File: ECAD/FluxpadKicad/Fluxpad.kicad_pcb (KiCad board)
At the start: 2 copper layers, 39 x 60 mm, 26 parts, among them SW1 SW_SPST, SW2 SW_SPST, SW3 PEC12R-4017F-N0024, U1 SeeeduinoXIAO, U2 DRV5056A3QDBZx Lekker, U3 DRV5056A3QDBZx Lekker

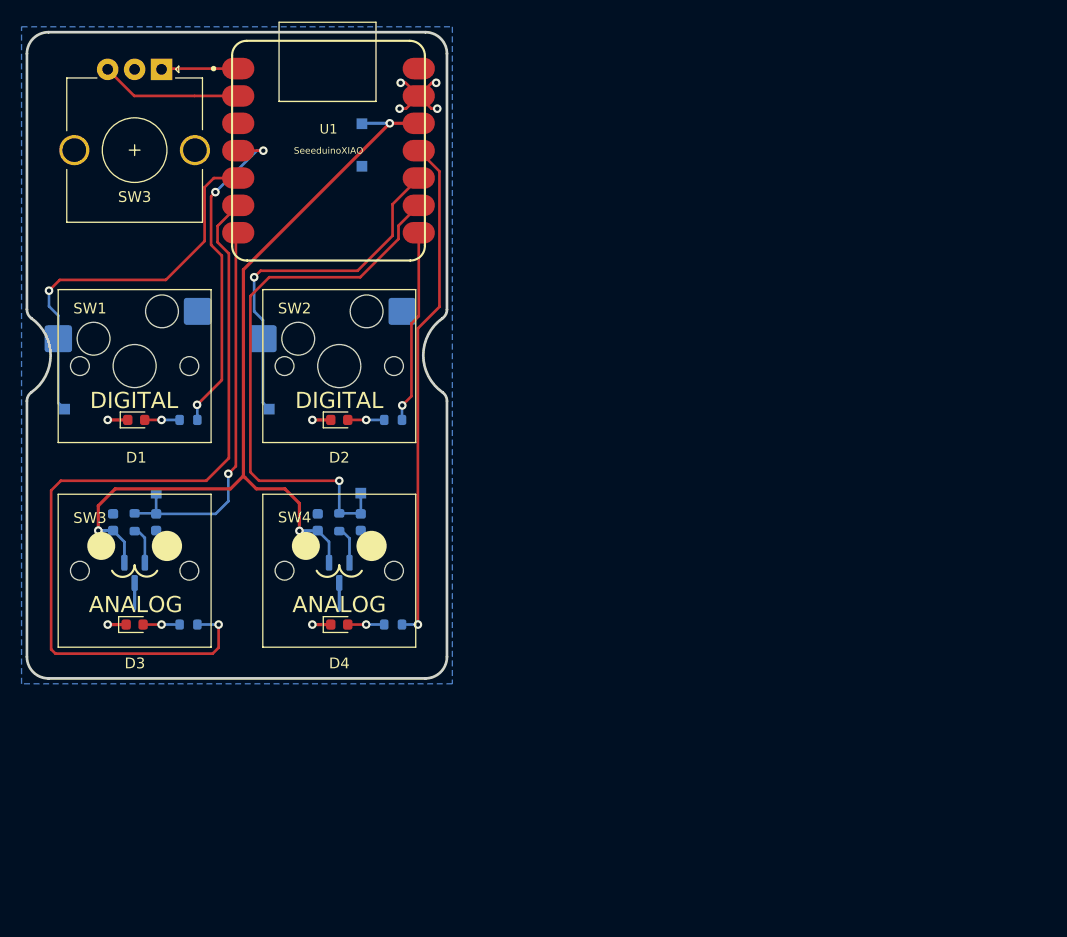
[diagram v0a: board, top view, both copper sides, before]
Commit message: initial commit for fluxpad 2
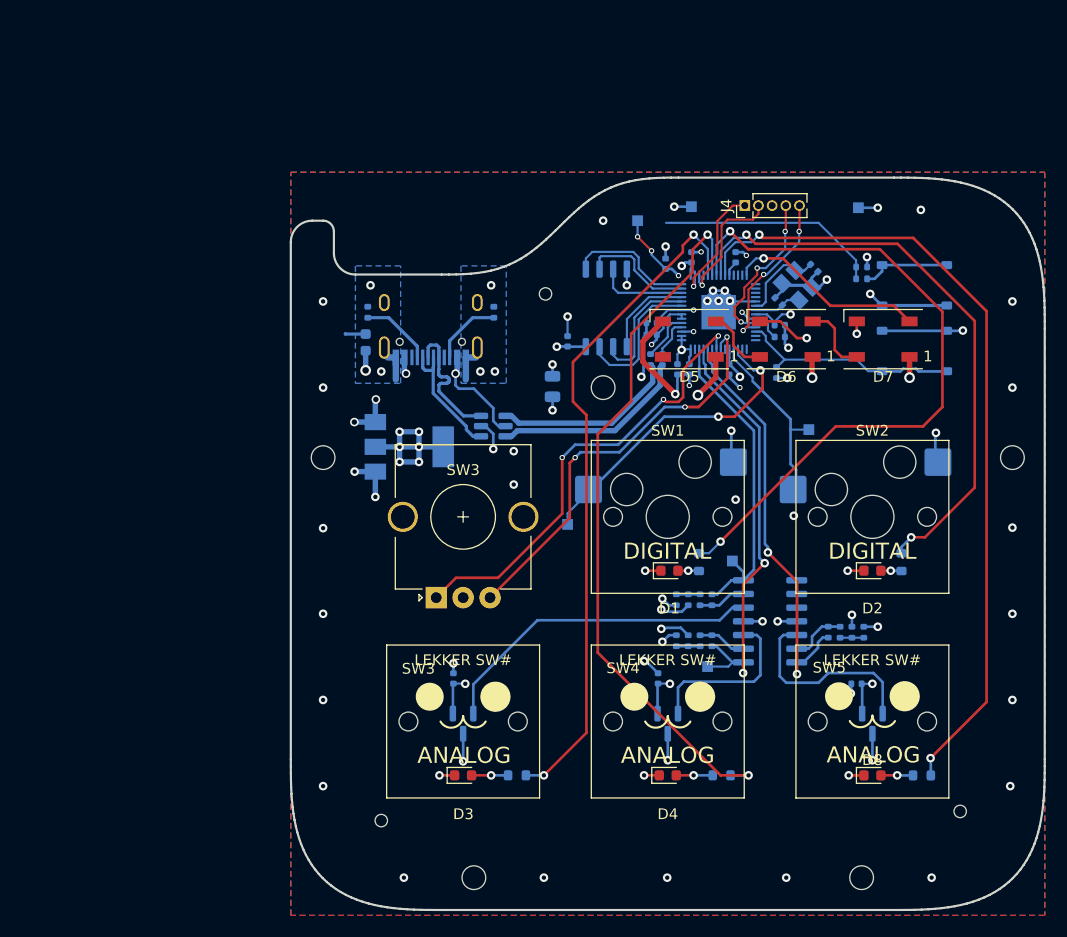
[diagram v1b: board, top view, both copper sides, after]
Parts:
- removed C3, C4: DNP, Capacitor_SMD:C_0603_1608Metric
- added 1V1: TestPoint, TestPoint:TestPoint_Pad_1.0x1.0mm, B.Cu at (157.2, 82.5)
- added C11: 100n, Capacitor_SMD:C_0402_1005Metric, B.Cu at (166.3, 85.9)
- added C12: 100n, Capacitor_SMD:C_0402_1005Metric, B.Cu at (165.7, 96.3)
- added C14: 100n, Capacitor_SMD:C_0402_1005Metric, B.Cu at (170.4, 92.2)
- added C15: 100n, Capacitor_SMD:C_0402_1005Metric, B.Cu at (170.4, 93.3)
- added C16: 100n, Capacitor_SMD:C_0402_1005Metric, B.Cu at (158.5, 92.0)
- added C17: 1u, Capacitor_SMD:C_0402_1005Metric, B.Cu at (159.8, 86.5)
- added C18: 1u, Capacitor_SMD:C_0402_1005Metric, B.Cu at (150.7, 93.7)
- added C19: 100n, Capacitor_SMD:C_0402_1005Metric, B.Cu at (158.5, 93.1)
- added C20: 30p, Capacitor_SMD:C_0402_1005Metric, B.Cu at (170.3, 90.0)
- added C21: 30p, Capacitor_SMD:C_0402_1005Metric, B.Cu at (173.6, 86.9)
- added C22: 1uF, Capacitor_SMD:C_0402_1005Metric, B.Cu at (177.5, 125.5)
- added C5: 22uf, Capacitor_SMD:C_0805_2012Metric, B.Cu at (149.3, 97.9)
- added C6: 10uf, Capacitor_SMD:C_0603_1608Metric, B.Cu at (131.9, 93.8)
- added C7: 100n, Capacitor_SMD:C_0402_1005Metric, B.Cu at (160.9, 96.3)
- added C8: 100n, Capacitor_SMD:C_0402_1005Metric, B.Cu at (162.2, 85.9)
- added C9: 100n, Capacitor_SMD:C_0402_1005Metric, B.Cu at (162.0, 96.3)
- added D5: WS2812B, LED_SMD:LED_WS2812B_PLCC4_5.0x5.0mm_P3.2mm, F.Cu at (162.0, 93.5)
- added D6: WS2812B, LED_SMD:LED_WS2812B_PLCC4_5.0x5.0mm_P3.2mm, F.Cu at (171.0, 93.5)
- added D7: WS2812B, LED_SMD:LED_WS2812B_PLCC4_5.0x5.0mm_P3.2mm, F.Cu at (180.0, 93.5)
- added D8: WHITE LED, LED_SMD:LED_0603_1608Metric, F.Cu at (179.0, 134.0)
- added H1: MountingHole, MountingHole:MountingHole_2.2mm_M2_ISO7380, F.Cu at (128.0, 104.5)
- added H2: MountingHole, MountingHole:MountingHole_2.2mm_M2_ISO7380, F.Cu at (142.0, 143.5)
- added H3: MountingHole, MountingHole:MountingHole_2.2mm_M2_ISO7380, F.Cu at (178.0, 143.5)
- added H4: MountingHole, MountingHole:MountingHole_2.2mm_M2_ISO7380, F.Cu at (192.0, 104.5)
- added H5: MountingHole, MountingHole:MountingHole_2.2mm_M2_ISO7380, F.Cu at (154.0, 98.0)
- added H6: Tooling Hole, Tang:JLC Tooling Hole, F.Cu at (148.7, 89.3)
- added H7: Tooling Hole, Tang:JLC Tooling Hole, F.Cu at (133.4, 138.2)
- added H8: Tooling Hole, Tang:JLC Tooling Hole, F.Cu at (187.2, 137.3)
- added J1: USB_C_Receptacle_USB2.0, Tang:USB_C_Receptacle_HRO_TYPE-C-31-M-12, B.Cu at (138.0, 91.2)
- added J4: DEBUG, Connector_PinHeader_1.27mm:PinHeader_1x05_P1.27mm_Vertical, F.Cu at (167.2, 81.1)
- added R10: 10k, Resistor_SMD:R_0402_1005Metric, B.Cu at (178.0, 86.8)
- added R11: 22, Resistor_SMD:R_0402_1005Metric, B.Cu at (158.4, 95.4)
- added R12: 22, Resistor_SMD:R_0402_1005Metric, B.Cu at (159.5, 95.4)
- added R13: 1k, Resistor_SMD:R_0402_1005Metric, B.Cu at (178.0, 87.9)
- added R14: 820R, Resistor_SMD:R_0402_1005Metric, B.Cu at (160.8, 121.5)
- added R15: 22, Resistor_SMD:R_0603_1608Metric, B.Cu at (183.6, 134.0)
- added R16: 820R, Resistor_SMD:R_0402_1005Metric, B.Cu at (160.8, 117.7)
- added R17: 5.6K, Resistor_SMD:R_0402_1005Metric, B.Cu at (163.0, 117.7)
- added R18: 10K, Resistor_SMD:R_0402_1005Metric, B.Cu at (164.1, 117.7)
- added R19: 220R, Resistor_SMD:R_0402_1005Metric, B.Cu at (177.1, 120.7)
- added R20: 820R, Resistor_SMD:R_0402_1005Metric, B.Cu at (178.2, 120.7)
- added R21: 5.6K, Resistor_SMD:R_0402_1005Metric, B.Cu at (163.0, 121.5)
- added R22: 5.6K, Resistor_SMD:R_0402_1005Metric, B.Cu at (176.0, 120.7)
- added R23: 10K, Resistor_SMD:R_0402_1005Metric, B.Cu at (164.1, 121.5)
- added R24: 10K, Resistor_SMD:R_0402_1005Metric, B.Cu at (174.9, 120.7)
- added R7: 5.1k, Resistor_SMD:R_0402_1005Metric, B.Cu at (132.2, 91.0)
- added R8: 5.1k, Resistor_SMD:R_0402_1005Metric, B.Cu at (143.8, 91.0)
- added R9: 10k, Resistor_SMD:R_0402_1005Metric, B.Cu at (170.1, 96.6)
- added SW4: RESET, Tang:SPST SMD TS-1187A-B-A-B, B.Cu at (182.9, 94.6)
- added SW5: BOOTSEL, Tang:SPST SMD TS-1187A-B-A-B, B.Cu at (182.9, 88.5)
- added SW6: SW_SPST, Tang:Kailh Hot Swap Socket, B.Cu at (159.4, 106.2)
- added SW7: SW_SPST, Tang:Kailh Hot Swap Socket, B.Cu at (178.4, 106.2)
- added U4: RP2040, Package_DFN_QFN:QFN-56-1EP_7x7mm_P0.4mm_EP3.2x3.2mm, B.Cu at (164.7, 91.0)
- added U5: DRV5056A3QDBZx Lekker, Tang:SW_Cherry_MX_PCB_1.00u_hall_effect, B.Cu at (179.0, 129.0)
- added U6: W25Q128JVS, Tang:SOIC-8_5.23x5.23mm_P1.27mm, B.Cu at (154.3, 90.6)
- added U7: USBLC6-2SC6, Package_TO_SOT_SMD:SOT-23-6, B.Cu at (143.8, 101.6)
- added U8: AMS1117-3.3, Package_TO_SOT_SMD:SOT-223-3_TabPin2, B.Cu at (136.0, 103.5)
- added Y1: Crystal_GND24, Crystal:Crystal_SMD_3225-4Pin_3.2x2.5mm, B.Cu at (172.0, 88.5)
- C1, C2: value 0.1uF -> 1uF; footprint Capacitor_SMD:C_0603_1608Metric -> Capacitor_SMD:C_0402_1005Metric
- D1, D2, D3, D4: value LED -> WHITE LED
- R1, R2, R3, R4: value 20 -> 22
- R5, R6: value 0 -> 220R; footprint Resistor_SMD:R_0603_1608Metric -> Resistor_SMD:R_0402_1005Metric
- SW1, SW2: footprint Switch_Keyboard_Hotswap_Kailh:SW_Hotswap_Kailh_MX_1.00u -> Tang:SW_Hotswap_Kailh_MX_no_pads
- U1: value SeeeduinoXIAO -> LM324A; footprint Tang:Seeeduino XIAO-MOUDLE14P-2.54-21X17.8MM -> Package_SO:SOIC-14_3.9x8.7mm_P1.27mm; moved to B.Cu
- moved U1 59.9 mm to (169.5, 119.7), turned to 180 degrees
- moved SW3 55.3 mm to (138.5, 117.5), turned to 90 degrees
- moved TP_SW3 53.9 mm to (166.0, 114.1)
- moved R5 51.9 mm to (161.9, 117.7)
- moved D1 51.4 mm to (160.2, 115.0)
- moved D2 51.4 mm to (179.0, 115.0)
- moved SW1 51.4 mm to (160.0, 110.0)
- moved SW2 51.4 mm to (179.0, 110.0)
- moved TP_SW2 50.1 mm to (173.1, 101.9)
- moved R1 49.2 mm to (162.9, 114.2), turned to 90 degrees
- moved R2 49.0 mm to (181.7, 114.2), turned to 90 degrees
- moved TP_SW1 47.9 mm to (150.7, 110.7)
- moved 3V3 46.8 mm to (177.7, 81.3)
- moved TP_SW4 36.0 mm to (163.7, 123.9)
- moved C1 34.8 mm to (140.1, 125.0)
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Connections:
- C1 pad 1: +3V3 -> +5V
- C2 pad 1: +3V3 -> +5V
- R1 pad 2: LED1 -> /LED1
- R2 pad 2: LED2 -> /LED2
- R3 pad 2: LED3 -> /LED3
- R4 pad 2: LED4 -> /LED4
- R5 pad 1: Net-(R5-Pad1) -> +5V
- R5 pad 2: SW3 -> Net-(R16-Pad2)
- R6 pad 1: Net-(R6-Pad1) -> +5V
- R6 pad 2: SW4 -> Net-(R14-Pad2)
- SW3 pad A: ENCA -> /ENCA
- SW3 pad B: ENCB -> /ENCB
- U1 pad 1: ENCA -> unconnected-(U1-Pad1)
- U1 pad 10: SW2 -> Net-(U1C-+)
- U1 pad 11: LED4 -> GND
- U1 pad 12: +3V3 -> Net-(U1D-+)
- U1 pad 13: GND -> Net-(U1D--)
- U1 pad 14: +5V -> SW3
- U1 pad 2: ENCB -> unconnected-(U1A---Pad2)
- U1 pad 4: LED1 -> +5V
- U1 pad 5: SW1 -> Net-(U1B-+)
- U1 pad 6: LED3 -> Net-(U1B--)
- U1 pad 7: SW3 -> /SW5
- U1 pad 8: LED2 -> SW4
- U1 pad 9: SW4 -> Net-(U1C--)
- U2 pad 1: +3V3 -> +5V
- U2 pad 2: Net-(R5-Pad1) -> Net-(U1D-+)
- U3 pad 1: +3V3 -> +5V
- U3 pad 2: Net-(R6-Pad1) -> Net-(U1C-+)
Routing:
- net +5V: track 0.00 -> 188.1 mm, vias 0 -> 15
- net GND: track 20.4 -> 113.4 mm, vias 8 -> 66
- net LED3: track 77.2 -> 0.00 mm, vias 1 -> 0
- net /LED5: track 0.00 -> 75.3 mm, vias 0 -> 2
- net /LED4: track 0.00 -> 67.4 mm, vias 0 -> 2
- net /LED1: track 0.00 -> 64.3 mm, vias 0 -> 2
- net /LED3: track 0.00 -> 63.0 mm, vias 0 -> 2
- net /LED2: track 0.00 -> 54.9 mm, vias 0 -> 2
- net LED4: track 47.0 -> 0.00 mm, vias 1 -> 0
- net /ENCA: track 0.00 -> 42.3 mm, vias 0 -> 3
- net /SW5: track 0.00 -> 38.9 mm, vias 0 -> 2
- net /ENCB: track 0.00 -> 38.7 mm, vias 0 -> 3
- net /QSPI_SS: track 0.00 -> 32.8 mm
- net LED1: track 31.1 -> 0.00 mm, vias 3 -> 0
- net Net-(U1D-+): track 0.00 -> 30.7 mm
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- added copper zone on In1.Cu, net +3V3
- added copper zone on In1.Cu, net +5V
- added copper zone on F.Cu, net GND
- added copper zone on In2.Cu, net GND
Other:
- board size 39 x 60 mm -> 70 x 68 mm
- copper layers 2 -> 4
- board text added: "FLUXPAD RevA T.W."
- board text removed: "FLUXPAD Rev3 T.W."
